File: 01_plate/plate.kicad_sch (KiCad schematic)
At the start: 62 parts, among them U1 HOLE, U10 HOLE, U11 HOLE, U12 HOLE, U13 HOLE, U14 HOLE, U15 HOLE, U16 HOLE, U17 HOLE, U18 HOLE, U19 HOLE, U2 HOLE, U20 HOLE, U21 HOLE, U22 HOLE, U23 HOLE, U24 HOLE, U25 HOLE, U26 HOLE, U27 HOLE, U28 HOLE, U29 HOLE, U3 HOLE, U30 HOLE, U31 HOLE, U32 HOLE, U33 HOLE, U34 HOLE, U35 HOLE, U36 HOLE, U37 HOLE, U38 HOLE, U39 HOLE, U4 HOLE, U40 HOLE, U41 HOLE, U42 HOLE, U43 HOLE, U44 HOLE, U45 HOLE, U46 HOLE, U47 HOLE, U48 HOLE, U49 HOLE, U5 HOLE, U50 HOLE, U51 HOLE, U52 HOLE, U53 HOLE, U54 HOLE, U55 HOLE, U56 HOLE, U57 HOLE, U58 HOLE, U59 HOLE, U6 HOLE, U60 HOLE, U67 HOLE, U7 HOLE, U8 HOLE, U9 HOLE

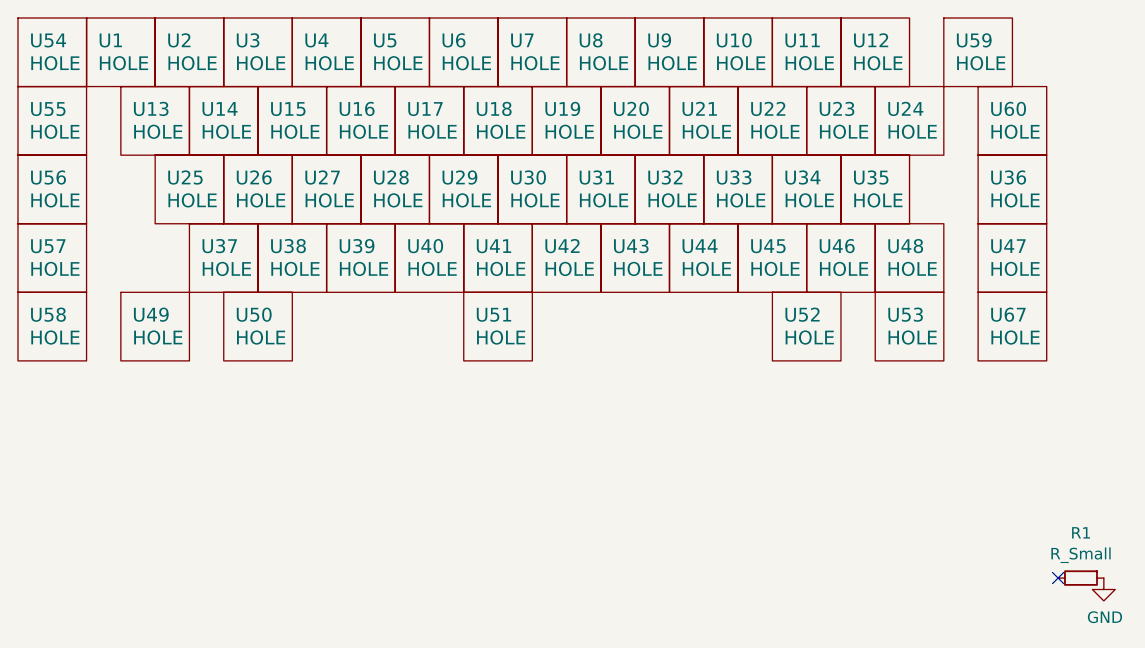
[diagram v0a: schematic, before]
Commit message: FR4 plate
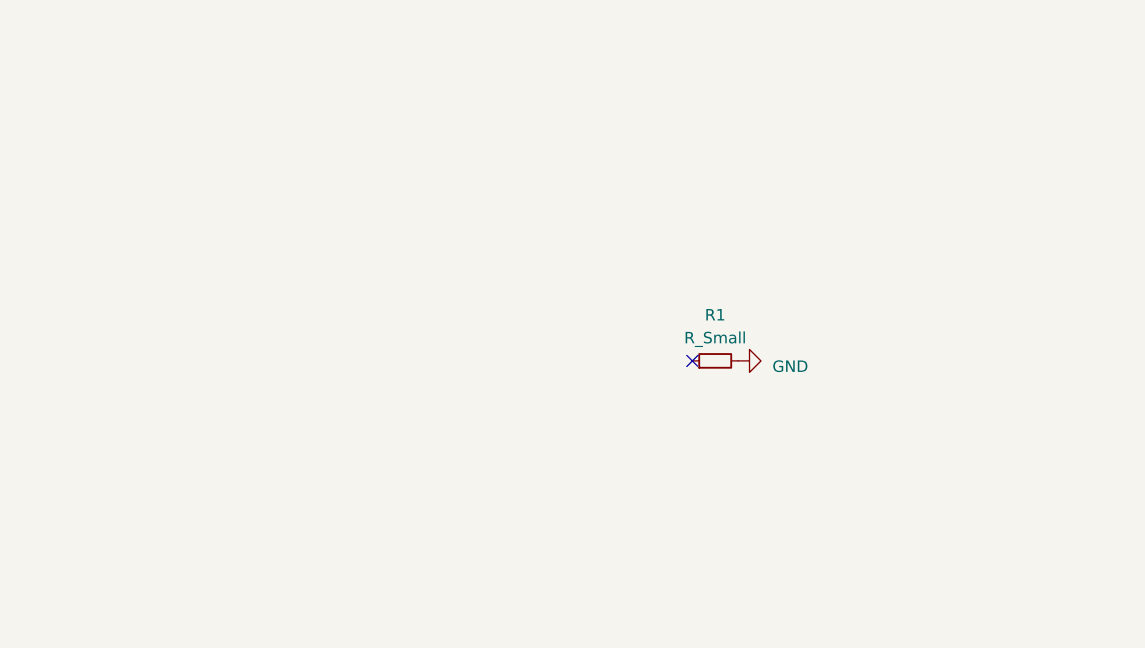
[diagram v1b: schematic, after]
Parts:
- removed U1, U10, U11, U12, U13, U14, U15, U16, U17, U18, U19, U2, U20, U21, U22, U23, U24, U25, U26, U27, U28, U29, U3, U30, U31, U32, U33, U34, U35, U37, U38, U39, U4, U40, U41, U42, U43, U44, U45, U46, U47, U49, U5, U53, U54, U6, U7, U8, U9: HOLE, Keeb_footprints:MX_100_cutout, symbol lets_split-cache:HOLE
- removed U36, U57: HOLE, Keeb_footprints:MX_225_cutout, symbol lets_split-cache:HOLE
- removed U48, U56: HOLE, Keeb_footprints:MX_175_cutout, symbol lets_split-cache:HOLE
- removed U50, U52, U55, U58, U60, U67: HOLE, Keeb_footprints:MX_150_cutout, symbol lets_split-cache:HOLE
- removed U51: HOLE, Keeb_footprints:MX_700_cutout, symbol lets_split-cache:HOLE
- removed U59: HOLE, Keeb_footprints:MX_200_cutout, symbol lets_split-cache:HOLE
- R1: footprint Resistor_SMD:R_0603_1608Metric_Pad1.05x0.95mm_HandSolder -> Resistor_SMD:R_0402_1005Metric
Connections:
- net GND: now also R1.2; no longer R1.1
